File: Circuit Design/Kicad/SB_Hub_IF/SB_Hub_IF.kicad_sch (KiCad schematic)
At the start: 55 parts, among them J1 POWER, J2 COMPUTER, U1 MCP23008-xSO

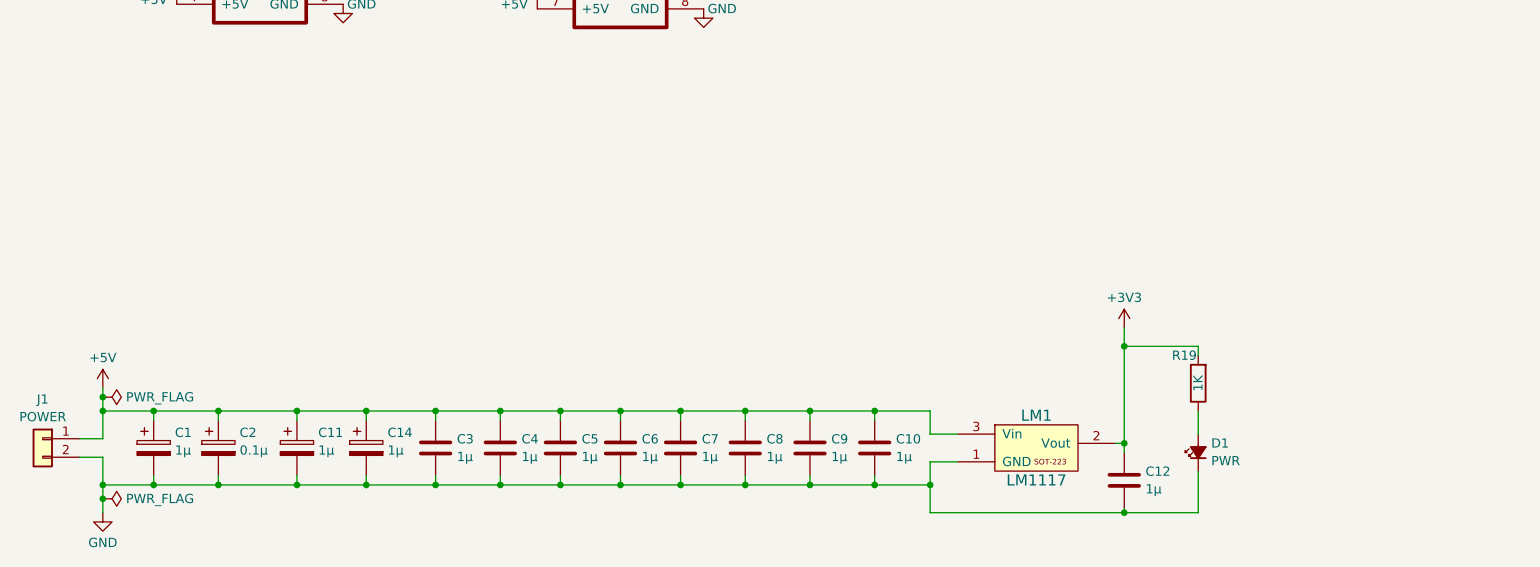
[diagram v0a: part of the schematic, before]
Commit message: Tidy up
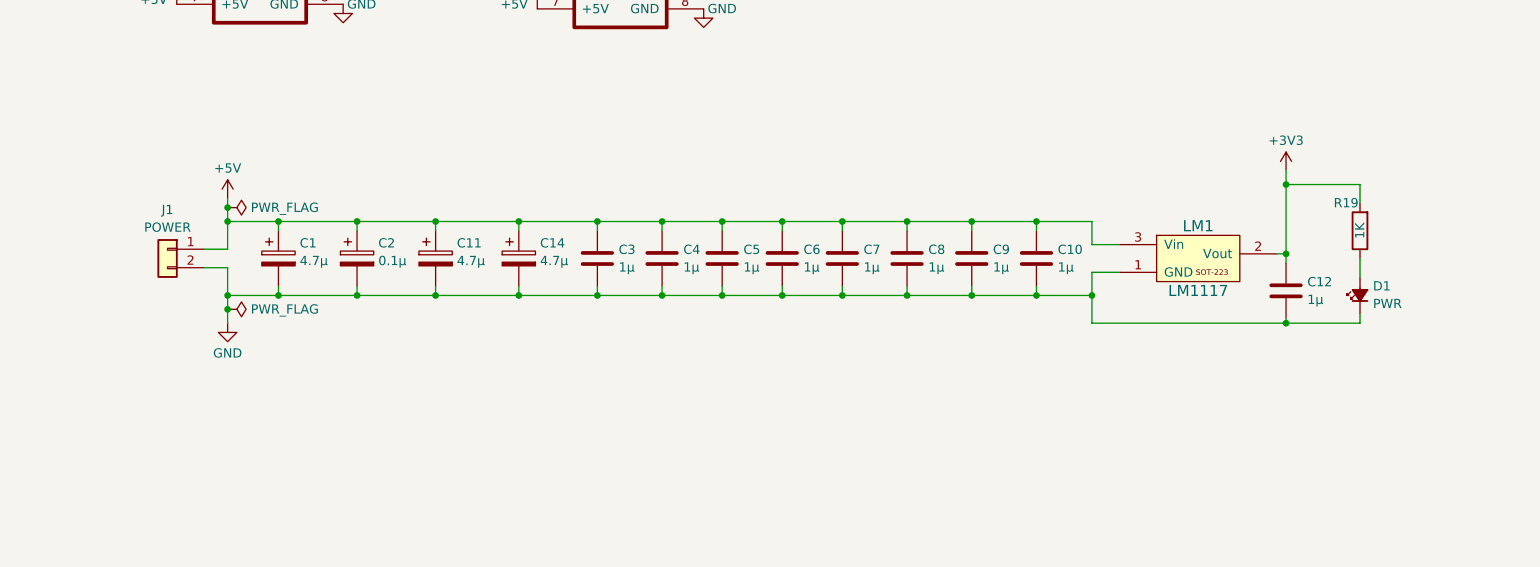
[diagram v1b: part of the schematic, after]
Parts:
- C1, C11, C14: value 1µ -> 4.7µ
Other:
- moved on the sheet: C1, C10, C11, C12, C14, C2, C3, C4, C5, C6, C7, C8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
